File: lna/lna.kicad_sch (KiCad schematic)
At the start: 12 parts, among them J1 Conn_Coaxial, J2 V5-GND, U1 PGA-103+

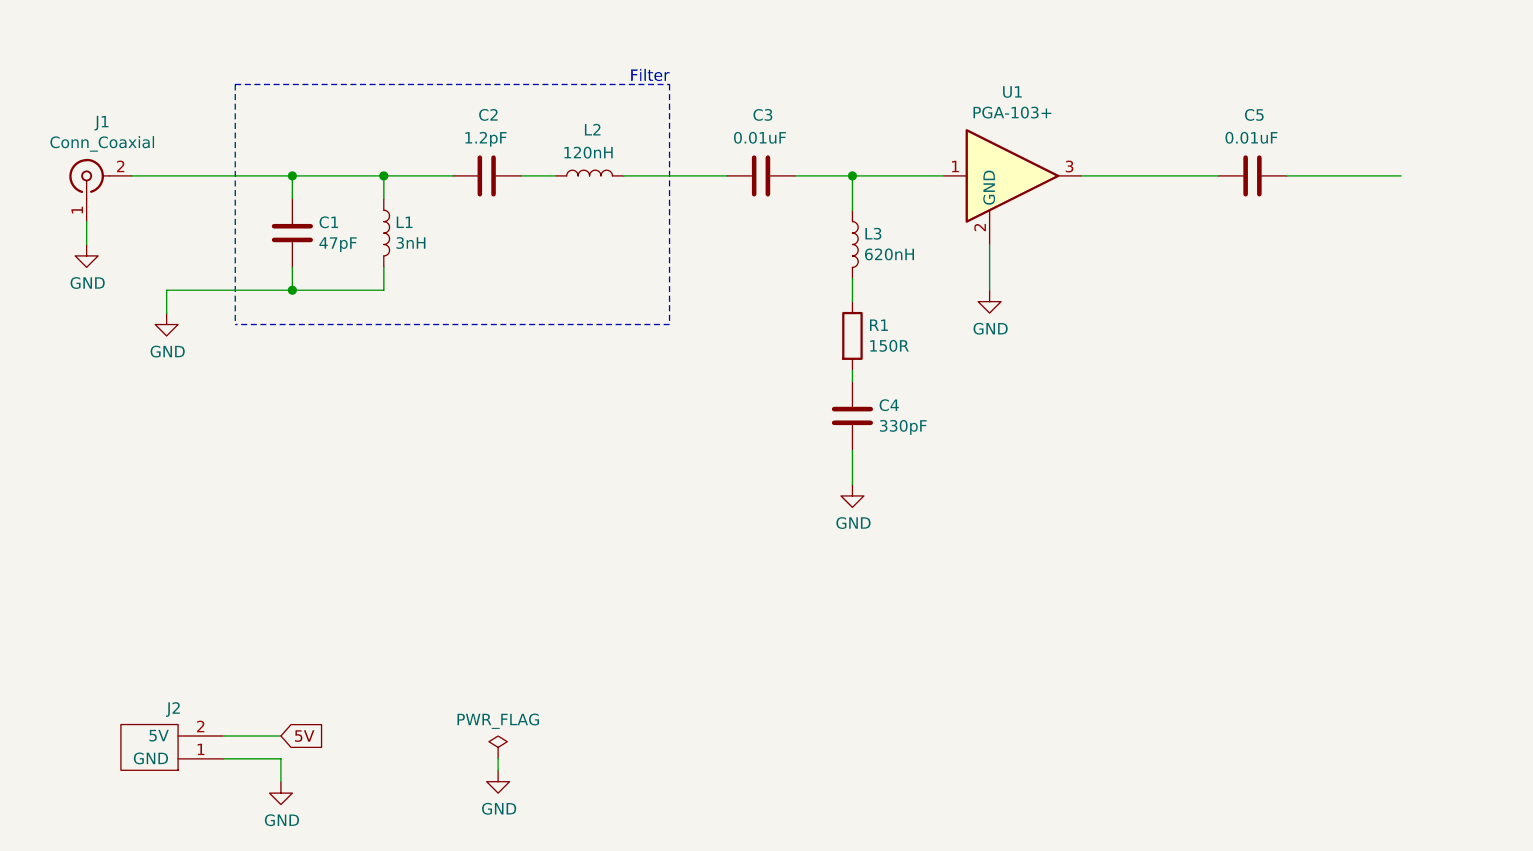
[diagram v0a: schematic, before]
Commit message: Schematics
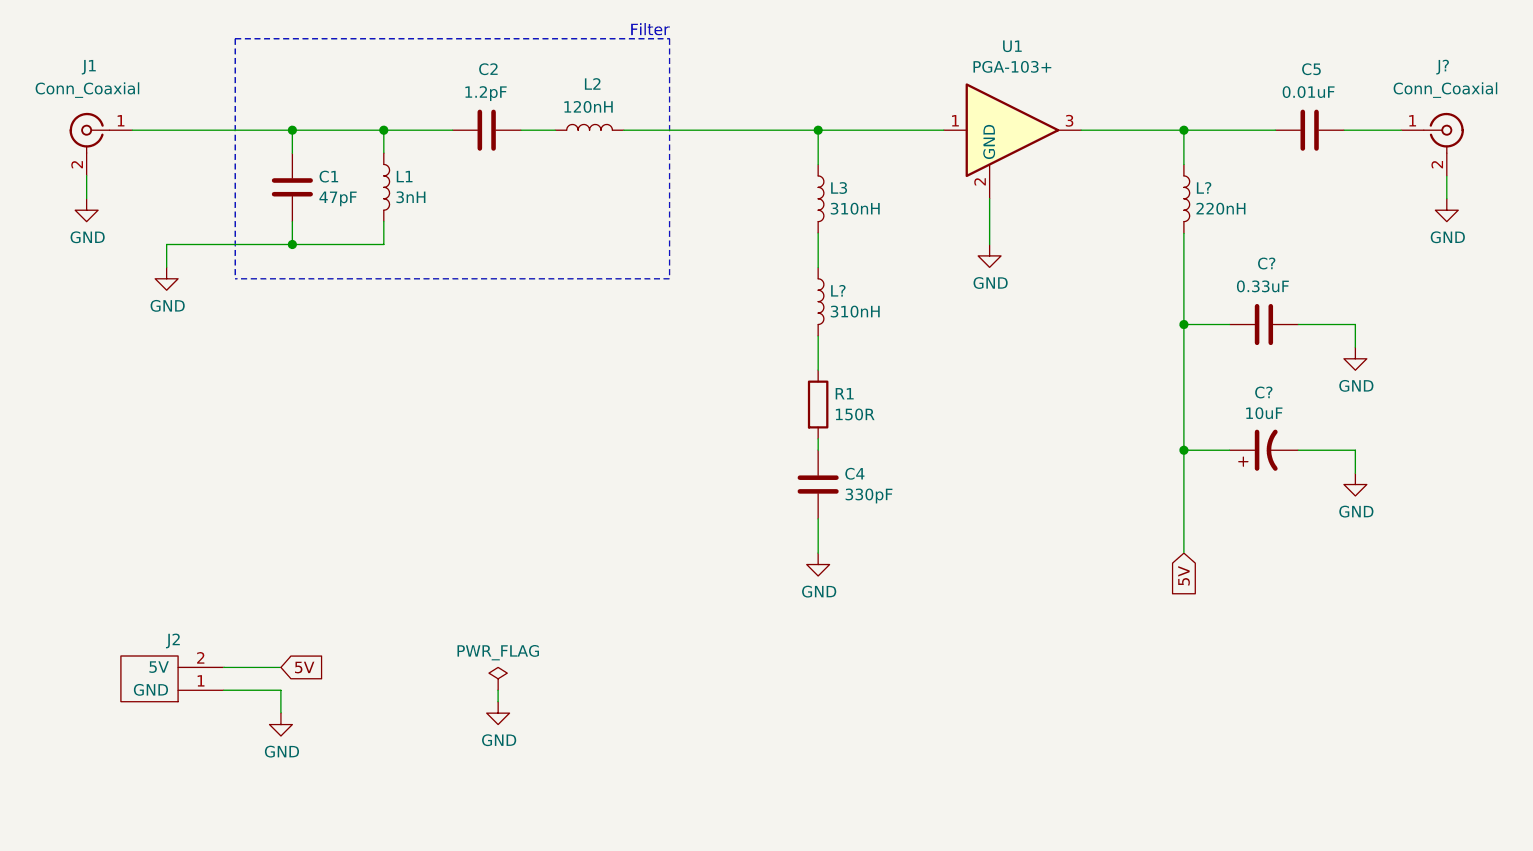
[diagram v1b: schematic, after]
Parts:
- removed C3: 0.01uF, symbol Device:C
- added C?: 0.33uF, symbol Device:C
- added C?: 10uF, symbol Device:CP1
- added J?: Conn_Coaxial, symbol Connector:Conn_Coaxial
- added L?: 220nH, symbol Device:L
- added L?: 310nH, symbol Device:L
- L3: value 620nH -> 310nH
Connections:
- net 5V: now also C?.1, C?.1, L?.2
- net GND: now also J1.2 (Ext), C?.2, C?.2, J?.2 (Ext); no longer J1.1 (In)
- net at C1.1, C2.1, L1.1: now also J1.1 (In); no longer J1.2 (Ext)
- net at R1.1: now also L?.2; no longer L3.2
- net at L2.2: now also L3.1, U1.1
- net at C5.1, U1.3: now also L?.1
- net at C5.2: now also J?.1 (In)
- new net: L3.2, L?.1
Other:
- moved on the sheet: C1, C2, C4, C5, J1, J2, L1, L2, L3, R1, U1
